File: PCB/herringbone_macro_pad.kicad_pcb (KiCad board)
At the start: 2 copper layers, 114.3 x 114.3 mm, 33 parts, among them J1 Screw_Terminal_01x04, SW1 CherryMX_2.75u_PCB_StabWireBo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, SW10 CherryMX_1.00u_PCB, SW11 SW_Push, SW2 CherryMX_1.00u_PCB, SW3 CherryMX_2.75u_PCB_StabWireBo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, SW4 CherryMX_2.75u_PCB_StabWireBo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, SW5 CherryMX_1.00u_PCB, SW6 CherryMX_2.75u_PCB_StabWireBo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, SW7 CherryMX_2.75u_PCB_StabWireBo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, SW8 CherryMX_1.00u_PCB, SW9 CherryMX_2.75u_PCB_StabWireBo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, U1 SRV05-4, U2 AMS1117, U3 STM32L151C8TxA, Y1 Crystal

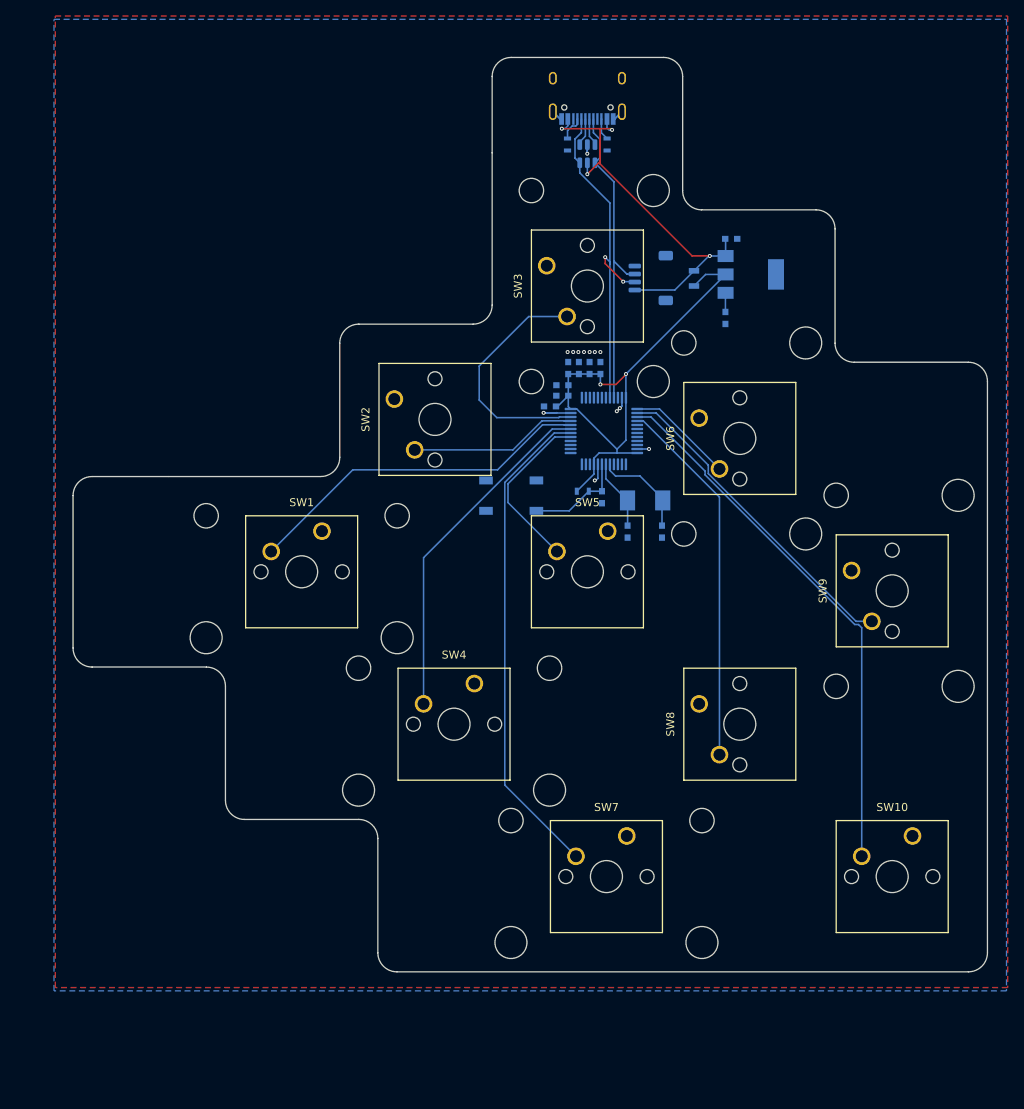
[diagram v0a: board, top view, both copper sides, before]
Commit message: Hardware revision.
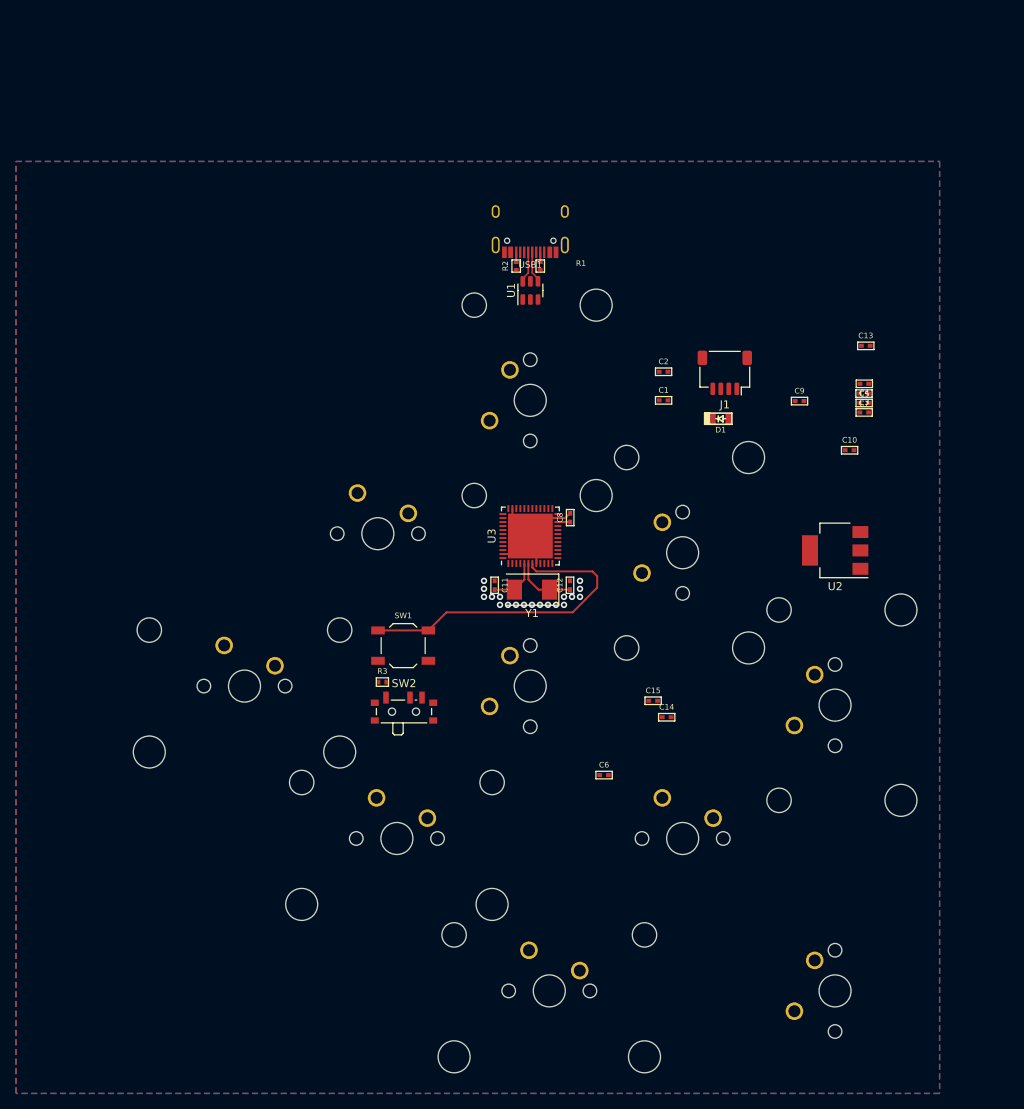
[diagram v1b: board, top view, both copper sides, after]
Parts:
- removed R5: 10k, Keebio-Parts:R_0603
- added C13: 0.1u, Keebio-Parts:C_0402, F.Cu at (196.7, 64.6)
- added C14: 0.1u, Keebio-Parts:C_0402, F.Cu at (171.8, 111.0)
- added C15: 0.1u, Keebio-Parts:C_0402, F.Cu at (170.1, 109.0)
- added R3: 10k, Keebio-Parts:R_0402, F.Cu at (136.3, 106.7)
- added SW12: CherryMX_2.75u_PCB_StabWireBottom, Button_Switch_Keyboard:SW_Cherry_MX_2.75u_PCB, B.Cu at (116.5, 102.1)
- C1: value 22p -> 22u; footprint Keebio-Parts:C_0603 -> Keebio-Parts:C_0402; moved to F.Cu
- C10: value 10n -> 0.1u; footprint Keebio-Parts:C_0603 -> Keebio-Parts:C_0402; moved to F.Cu
- C11: value 1u -> 30p; footprint Keebio-Parts:C_0603 -> Keebio-Parts:C_0402; moved to F.Cu
- C12: value 0.1u -> 30p; footprint Keebio-Parts:C_0603 -> Keebio-Parts:C_0402; moved to F.Cu
- C2: value 22p -> 10u; footprint Keebio-Parts:C_0603 -> Keebio-Parts:C_0402; moved to F.Cu
- C3: value 22u -> 4.7u; footprint Keebio-Parts:C_0603 -> Keebio-Parts:C_0402; moved to F.Cu
- C4: value 10u -> 4.7u; footprint Keebio-Parts:C_0603 -> Keebio-Parts:C_0402; moved to F.Cu
- C5: value 4.7u -> 0.1u; footprint Keebio-Parts:C_0603 -> Keebio-Parts:C_0402; moved to F.Cu
- C6, C7, C9: value 100n -> 0.1u; footprint Keebio-Parts:C_0603 -> Keebio-Parts:C_0402; moved to F.Cu
- C8: value 100n -> 4.7u; footprint Keebio-Parts:C_0603 -> Keebio-Parts:C_0402; moved to F.Cu
- D1, U1, U2, USB1, Y1: moved to F.Cu
- J1: value Screw_Terminal_01x04 -> JST; moved to F.Cu
- R1, R2: footprint Keebio-Parts:R_0603 -> Keebio-Parts:R_0402; moved to F.Cu
- SW1: value CherryMX_2.75u_PCB_StabWireBottom -> SW_Push; footprint CherryMX_PCB_StabWireBottom:CherryMX_2.75u_PCB_StabWireBottom -> Keebio-Parts:SW_SPST_TL3342
- SW10, SW5: value CherryMX_1.00u_PCB -> CherryMX_2.75u_PCB_StabWireBottom; footprint CherryMX_PCB:CherryMX_1.00u_PCB -> Button_Switch_Keyboard:SW_Cherry_MX_2.75u_PCB; moved to B.Cu
- SW11: value SW_Push -> CherryMX_1.00u_PCB; footprint Keebio-Parts:SW_SPST_TL3342 -> Button_Switch_Keyboard:SW_Cherry_MX_1.00u_PCB
- SW2: value CherryMX_1.00u_PCB -> SW_SPST; footprint CherryMX_PCB:CherryMX_1.00u_PCB -> Button_Switch_SMD:SW_SPDT_PCM12
- SW3, SW6, SW7: footprint CherryMX_PCB_StabWireBottom:CherryMX_2.75u_PCB_StabWireBottom -> Button_Switch_Keyboard:SW_Cherry_MX_2.75u_PCB; moved to B.Cu
- SW4, SW9: value CherryMX_2.75u_PCB_StabWireBottom -> CherryMX_1.00u_PCB; footprint CherryMX_PCB_StabWireBottom:CherryMX_2.75u_PCB_StabWireBottom -> Button_Switch_Keyboard:SW_Cherry_MX_1.00u_PCB; moved to B.Cu
- SW8: footprint CherryMX_PCB:CherryMX_1.00u_PCB -> Button_Switch_Keyboard:SW_Cherry_MX_1.00u_PCB; moved to B.Cu
- U3: value STM32L151C8TxA -> STM32F411CEUx; footprint Package_QFP:LQFP-48_7x7mm_P0.5mm -> Package_DFN_QFN:QFN-48-1EP_7x7mm_P0.5mm_EP5.6x5.6mm; moved to F.Cu
- moved SW10 76.0 mm to (149.7, 74.0), turned to -90 degrees
- moved SW6 63.9 mm to (135.6, 121.1), turned to 180 degrees
- moved SW9 53.9 mm to (187.8, 147.8), turned to -90 degrees
- moved C6 50.9 mm to (164.0, 118.3), turned to 0 degrees
- moved SW5 47.9 mm to (154.6, 140.2), turned to 180 degrees
- moved SW11 42.2 mm to (171.3, 121.1), turned to 180 degrees
- moved C5 37.8 mm to (196.5, 69.4)
- moved C7 37.7 mm to (196.5, 70.6)
- moved SW3 36.5 mm to (168.8, 93.0), turned to -90 degrees
- moved SW2 36.4 mm to (139.0, 110.0), turned to 0 degrees
- moved U2 36.1 mm to (192.9, 90.2), turned to 180 degrees
- moved C10 35.4 mm to (194.7, 77.7), turned to 0 degrees
- moved SW8 31.4 mm to (149.7, 109.7), turned to -90 degrees
- moved SW4 31.3 mm to (133.2, 83.0), turned to 180 degrees
- moved SW7 30.1 mm to (187.8, 112.1), turned to -90 degrees
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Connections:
- net /SW_8 renamed SW_3
- net /SW_9 renamed SW_4
- C1 pad 1: GND -> +5V
- C1 pad 2: /CLK_IN -> GND
- C11 pad 1: +3.3VA -> GND
- C11 pad 2: GND -> /CLK_IN
- C12 pad 1: /RST -> /CLK_OUT
- C2 pad 1: /CLK_OUT -> Net-(C2-Pad1)
- C3 pad 1: +5V -> +3.3VA
- C4 pad 1: Net-(C4-Pad1) -> +3.3VA
- C8 pad 1: +3.3VA -> /V_CAP
- SW1 pad 1: /SW_0 -> /RST
- SW11 pad 1: /RST -> SW_10
- SW2 pad 1: /SW_5 -> Net-(R3-Pad2)
- SW2 pad 2: GND -> /BOOT
- SW3 pad 1: /SW_1 -> SW_1
- SW4 pad 1: /SW_6 -> SW_6
- SW5 pad 1: /SW_2 -> SW_7
- SW6 pad 1: /SW_7 -> SW_2
- SW7 pad 1: /SW_3 -> SW_8
- SW9 pad 1: /SW_4 -> SW_9
- U2 pad 1: Net-(C4-Pad1) -> Net-(C2-Pad1)
- U3 pad 17: /SW_2 -> unconnected-(U3-Pad17)
- U3 pad 18: /SW_3 -> SW_1
- U3 pad 19: /SW_6 -> SW_5
- U3 pad 20: /SW_0 -> SW_2
- U3 pad 21: /SW_5 -> unconnected-(U3-Pad21)
- U3 pad 22: /SW_1 -> /V_CAP
- U3 pad 37: /SW_7 -> unconnected-(U3-Pad37)
- U3 pad 38: /SW_4 -> unconnected-(U3-Pad38)
- U3 pad 41: unconnected-(U3-Pad41) -> SW_6
- U3 pad 42: unconnected-(U3-Pad42) -> SW_7
- U3 pad 43: unconnected-(U3-Pad43) -> SW_10
- U3 pad 44: unconnected-(U3-Pad44) -> /BOOT
- U3 pad 45: unconnected-(U3-Pad45) -> SW_9
- U3 pad 46: unconnected-(U3-Pad46) -> SW_8
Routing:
- net SW_4: track 67.8 -> 0.00 mm
- net +3.3VA: track 66.7 -> 0.00 mm, vias 2 -> 0
- net /SW_3: track 61.2 -> 0.00 mm
- net +5V: track 51.8 -> 0.00 mm, vias 4 -> 0
- net SW_3: track 46.4 -> 0.00 mm
- net /SW_0: track 44.0 -> 0.00 mm
- net /SW_6: track 43.3 -> 0.00 mm
- net /D1-: track 47.0 -> 3.91 mm, vias 2 -> 0
- net /SW_4: track 40.7 -> 0.00 mm
- net /D1+: track 43.2 -> 3.93 mm
- net /SW_1: track 30.2 -> 0.00 mm
- net /RST: track 12.6 -> 40.1 mm
- net /SW_2: track 21.2 -> 0.00 mm
- net /SW_5: track 21.0 -> 0.00 mm
- net /SW_7: track 13.4 -> 0.00 mm
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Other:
- board outline removed
